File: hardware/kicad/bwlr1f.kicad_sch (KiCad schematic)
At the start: 68 parts, among them J1 Conn_01x02, Q2 PMV32UP, Q3 DMG1012UW, U1 BME688, U1 RAK3172-SIP, U2 NBM7100ABQX, U3 ZD24C08A, U5 TPL5110

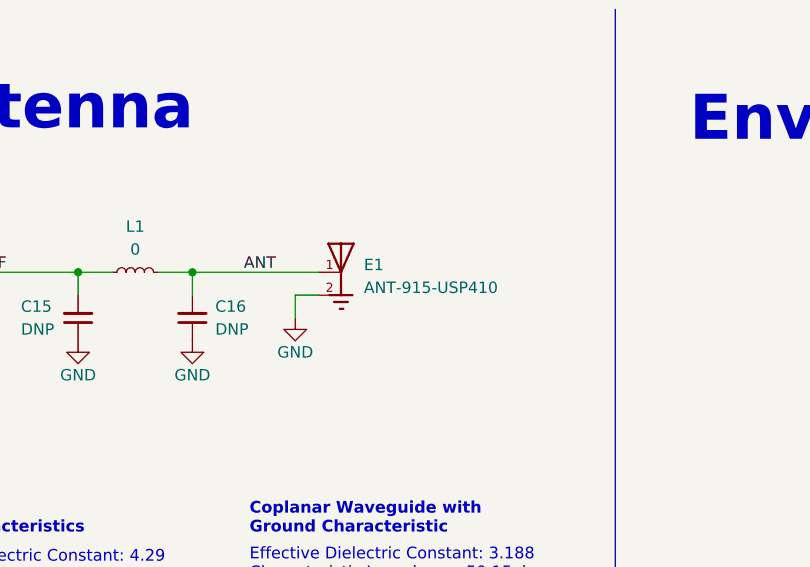
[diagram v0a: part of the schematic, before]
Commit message: change antenna
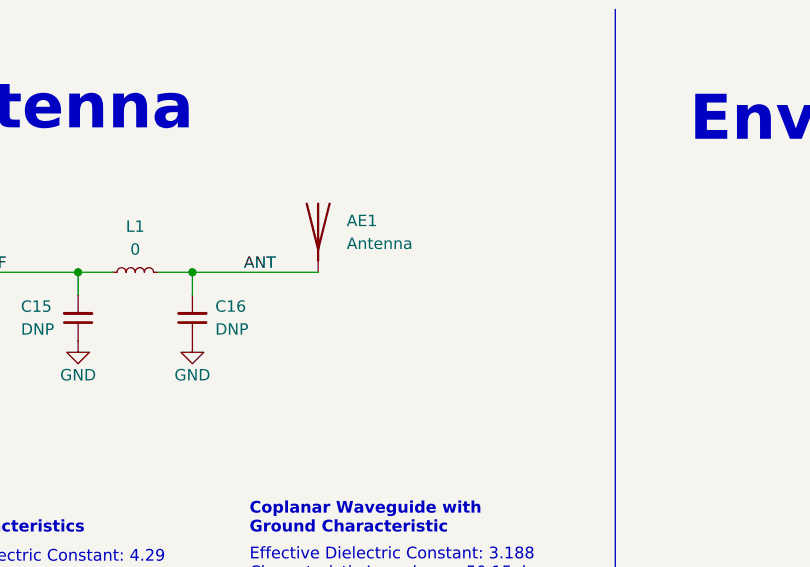
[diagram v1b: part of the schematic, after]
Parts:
- removed E1: ANT-915-USP410, bwlr1f:XDCR_ANT-915-USP410, symbol bwlr1f:ANT-915-USP410
- added AE1: Antenna, RF_Antenna:Texas_SWRA416_868MHz_915MHz, symbol Device:Antenna
- C15, C16: footprint Capacitor_SMD:C_0603_1608Metric -> Capacitor_SMD:C_0402_1005Metric
- L1: footprint Inductor_SMD:L_0603_1608Metric -> Inductor_SMD:L_0402_1005Metric; Distributor LCSC -> (none); Distributor Link https://www.lcsc.com/product-detail/Chip-Resistor-Surface-M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 -> (none); Distributor Part Number C21189 -> (none); Manufacturer UNI-ROYAL(Uniroyal Elec) -> (none); Manufacturer Part Number 0603WAF0000T5E -> (none); Part Description Resistors 100mW 75V ±1% 0Ω -> (none)
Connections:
- net ANT: now also AE1.1 (A)
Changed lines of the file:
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@@
     (stroke (width 0) (type default))
   )
-  (wire (pts (xy 243.84 45.72) (xy 243.84 43.18))
-    (stroke (width 0) (type default))
-  )
   (wire (pts (xy 44.45 43.18) (xy 44.45 41.91))
     (stroke (width 0) (type default))
   )
-  (wire (pts (xy 243.84 43.18) (xy 246.38 43.18))
-    (stroke (width 0) (type default))
-  )
   (wire (pts (xy 350.52 51.435) (xy 351.79 51.435))
     (stroke (width 0) (type default))
@@
     )
   )
+  (symbol (lib_id "Device:Antenna") (at 246.38 35.56 0) (unit 1)
+    (in_bom yes) (on_board yes) (dnp no) (fields_autoplaced)
+    (property "Reference" "AE1" (at 249.555 34.925 0)
+      (effects (font (size 1.27 1.27)) (justify left))
+    )
+    (property "Value" "Antenna" (at 249.555 37.465 0)
+      (effects (font (size 1.27 1.27)) (justify left))
+    )
+    (property "Footprint" "RF_Antenna:Texas_SWRA416_868MHz_915MHz" (at 246.38 35.56 0)
+      (effects (font (size 1.27 1.27)) hide)
+    )
+    (property "Datasheet" "~" (at 246.38 35.56 0)
+      (effects (font (size 1.27 1.27)) hide)
+    )
+    (property "Part Description" "" (at 246.38 35.56 0)
+      (effects (font (size 1.27 1.27)) hide)
+    )
+    (property "Manufacturer" "" (at 246.38 35.56 0)
+      (effects (font (size 1.27 1.27)) hide)
+    )
+    (property "Manufacturer Part Number" "" (at 246.38 35.56 0)
+      (effects (font (size 1.27 1.27)) hide)
+    )
+    (property "Distributor" "" (at 246.38 35.56 0)
+      (effects (font (size 1.27 1.27)) hide)
+    )
+    (property "Distributor Part Number" "" (at 246.38 35.56 0)
+      (effects (font (size 1.27 1.27)) hide)
+    )
+    (property "Distributor Link" "" (at 246.38 35.56 0)
+      (effects (font (size 1.27 1.27)) hide)
+    )
+    (pin "1")
+    (instances
+      (project "bwlr1f"
+        (path "/7fec048a-2dfd-4bff-8685-e805b00dfe07"
+          (reference "AE1") (unit 1)
+        )
+      )
+    )
+  )
   (symbol (lib_id "Device:C_Small") (at 232.41 45.72 180) (unit 1)
     (in_bom yes) (on_board yes) (dnp no) (fields_autoplaced)
@@
       (effects (font (size 1.27 1.27)) (justify right))
     )
-    (property "Footprint" "Capacitor_SMD:C_0603_1608Metric" (at 232.41 45.72 0)
+    (property "Footprint" "Capacitor_SMD:C_0402_1005Metric" (at 232.41 45.72 0)
       (effects (font (size 1.27 1.27)) hide)
     )
@@
       (effects (font (size 1.27 1.27)) hide)
     )
+    (property "Part Description" "" (at 232.41 45.72 0)
+      (effects (font (size 1.27 1.27)) hide)
+    )
+    (property "Manufacturer" "" (at 232.41 45.72 0)
+      (effects (font (size 1.27 1.27)) hide)
+    )
+    (property "Distributor" "" (at 232.41 45.72 0)
+      (effects (font (size 1.27 1.27)) hide)
+    )
+    (property "Distributor Part Number" "" (at 232.41 45.72 0)
+      (effects (font (size 1.27 1.27)) hide)
+    )
+    (property "Distributor Link" "" (at 232.41 45.72 0)
+      (effects (font (size 1.27 1.27)) hide)
+    )
     (pin "1")
     (pin "2")
@@
       (effects (font (size 1.27 1.27)))
     )
-    (property "Footprint" "Inductor_SMD:L_0603_1608Metric" (at 226.06 40.64 0)
-      (effects (font (size 1.27 1.27)) hide)
-    )
-    (property "Datasheet" "https://datasheet.lcsc.com/lcsc/2206010130_UNI-ROYAL-Uniroyal-Elec-0603WAF0000T5E_C21189.pdf" (at 226.06 40.64 0)
+    (property "Footprint" "Inductor_SMD:L_0402_1005Metric" (at 226.06 40.64 0)
       (effects (font (size 1.27 1.27)) hide)
     )
-    (property "Manufacturer Part Number" "0603WAF0000T5E" (at 226.06 40.64 0)
-      (effects (font (size 1.27 1.27)) hide)
-    )
-    (property "Part Description" "Resistors 100mW 75V ±1% 0Ω" (at 226.06 40.64 0)
-      (effects (font (size 1.27 1.27)) hide)
-    )
-    (property "Manufacturer" "UNI-ROYAL(Uniroyal Elec)" (at 226.06 40.64 0)
-      (effects (font (size 1.27 1.27)) hide)
-    )
-    (property "Distributor" "LCSC" (at 226.06 40.64 0)
-      (effects (font (size 1.27 1.27)) hide)
-    )
-    (property "Distributor Part Number" "C21189" (at 226.06 40.64 0)
-      (effects (font (size 1.27 1.27)) hide)
-    )
-    (property "Distributor Link" "https://www.lcsc.com/product-detail/Chip-Resistor-Surface-Mount_UNI-ROYAL-Uniroyal-Elec-0603WAF0000T5E_C21189.html" (at 226.06 40.64 0)
+    (property "Datasheet" "" (at 226.06 40.64 0)
       (effects (font (size 1.27 1.27)) hide)
     )
@@
       (effects (font (size 1.27 1.27)) (justify right))
     )
-    (property "Footprint" "Capacitor_SMD:C_0603_1608Metric" (at 219.71 45.72 0)
+    (property "Footprint" "Capacitor_SMD:C_0402_1005Metric" (at 219.71 45.72 0)
       (effects (font (size 1.27 1.27)) hide)
     )
@@
     )
   )
-  (symbol (lib_id "bwlr1f:ANT-915-USP410") (at 248.92 40.64 0) (unit 1)
-    (in_bom yes) (on_board yes) (dnp no) (fields_autoplaced)
-    (property "Reference" "E1" (at 251.46 39.8145 0)
-      (effects (font (size 1.27 1.27)) (justify left))
-    )
-    (property "Value" "ANT-915-USP410" (at 251.46 42.3545 0)
-      (effects (font (size 1.27 1.27)) (justify left))
-    )
-    (property "Footprint" "bwlr1f:XDCR_ANT-915-USP410" (at 243.84 50.8 0)
-      (effects (font (size 1.27 1.27)) (justify left bottom) hide)
-    )
-    (property "Datasheet" "https://www.te.com/commerce/DocumentDelivery/DDEController?Action=srchrtrv&DocNm=ant-915-usp410-ds&DocType=Data+Sheet&DocLang=English&DocFormat=pdf&PartCntxt=ANT-915-USP410" (at 248.92 40.64 0)
-      (effects (font (size 1.27 1.27)) (justify left bottom) hide)
-    )
-    (property "Part Description" "915MHz ISM, LoRaWAN, LPWA, Sigfox Chip RF Antenna 902MHz ~ 930MHz 0.9dBi Solder Surface Mount" (at 248.92 40.64 0)
-      (effects (font (size 1.27 1.27)) hide)
-    )
-    (property "Manufacturer" "TE Connectivity Linx" (at 248.92 40.64 0)
-      (effects (font (size 1.27 1.27)) hide)
-    )
-    (property "Manufacturer Part Number" "ANT-915-USP410" (at 248.92 40.64 0)
-      (effects (font (size 1.27 1.27)) hide)
-    )
-    (property "Distributor" "Digikey" (at 248.92 40.64 0)
-      (effects (font (size 1.27 1.27)) hide)
-    )
-    (property "Distributor Part Number" "343-ANT-915-USP410CT-ND" (at 248.92 40.64 0)
-      (effects (font (size 1.27 1.27)) hide)
-    )
-    (property "Distributor Link" "https://www.digikey.com/en/products/detail/te-connectivity-linx/ANT-915-USP410/13165344" (at 248.92 40.64 0)
-      (effects (font (size 1.27 1.27)) hide)
-    )
-    (pin "1")
-    (pin "2")
-    (instances
-      (project "bwlr1f"
-        (path "/7fec048a-2dfd-4bff-8685-e805b00dfe07"
-          (reference "E1") (unit 1)
-        )
-      )
-    )
-  )
   (symbol (lib_id "power:+3V0") (at 33.655 83.82 0) (unit 1)
     (in_bom yes) (on_board yes) (dnp no) (fields_autoplaced)
@@
         )
       )
-    )
-  )
-  (symbol (lib_id "power:GND") (at 243.84 45.72 0) (unit 1)
-    (in_bom yes) (on_board yes) (dnp no)
-    (property "Reference" "#PWR030" (at 243.84 52.07 0)
-      (effects (font (size 1.27 1.27)) hide)
-    )
-    (property "Value" "GND" (at 243.84 49.53 0)
-      (effects (font (size 1.27 1.27)))
-    )
-    (property "Footprint" "" (at 243.84 45.72 0)
-      (effects (font (size 1.27 1.27)) hide)
-    )
-    (property "Datasheet" "" (at 243.84 45.72 0)
-      (effects (font (size 1.27 1.27)) hide)
-    )
-    (pin "1")
-    (instances
-      (project "bwlr1e"
-        (path "/630c8da6-5464-4eef-824d-89618087f4b4"
-          (reference "#PWR030") (unit 1)
-        )
-      )
-      (project "bwlr1f"
-        (path "/7fec048a-2dfd-4bff-8685-e805b00dfe07"
-          (reference "#PWR038") (unit 1)
-        )
-      )

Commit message: Revert "change antenna"
This reverts commit 46c20b2a2dd1e0a5efdce99ceacd3ab7d772dc0d.
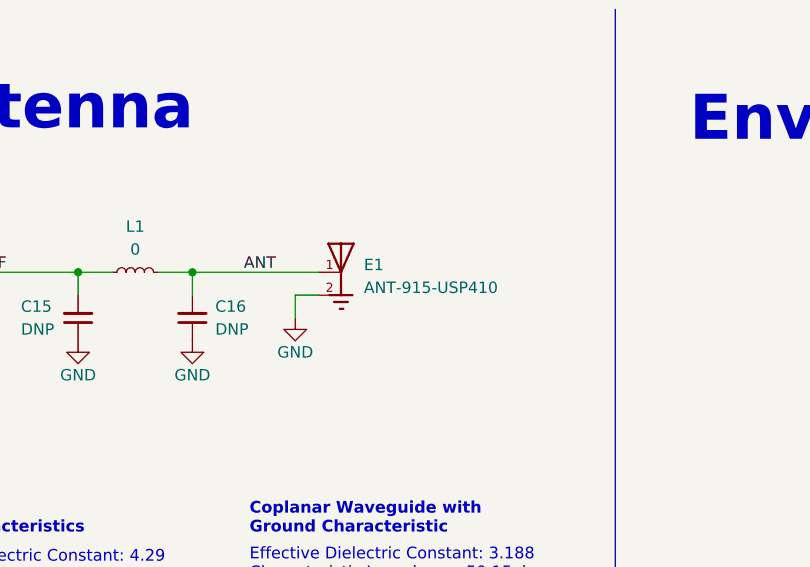
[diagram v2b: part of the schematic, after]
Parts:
- removed AE1: Antenna, RF_Antenna:Texas_SWRA416_868MHz_915MHz, symbol Device:Antenna
- added E1: ANT-915-USP410, bwlr1f:XDCR_ANT-915-USP410, symbol bwlr1f:ANT-915-USP410
- C15, C16: footprint Capacitor_SMD:C_0402_1005Metric -> Capacitor_SMD:C_0603_1608Metric
- L1: footprint Inductor_SMD:L_0402_1005Metric -> Inductor_SMD:L_0603_1608Metric; Distributor (none) -> LCSC; Distributor Link (none) -> https://www.lcsc.com/product-detail/Chip-Resistor-Surface-M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; Distributor Part Number (none) -> C21189; Manufacturer (none) -> UNI-ROYAL(Uniroyal Elec); Manufacturer Part Number (none) -> 0603WAF0000T5E; Part Description (none) -> Resistors 100mW 75V ±1% 0Ω
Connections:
- net ANT: now also E1.1
- net GND: now also E1.2
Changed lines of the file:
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@@
     (stroke (width 0) (type default))
   )
+  (wire (pts (xy 243.84 45.72) (xy 243.84 43.18))
+    (stroke (width 0) (type default))
+  )
   (wire (pts (xy 44.45 43.18) (xy 44.45 41.91))
     (stroke (width 0) (type default))
   )
+  (wire (pts (xy 243.84 43.18) (xy 246.38 43.18))
+    (stroke (width 0) (type default))
+  )
   (wire (pts (xy 350.52 51.435) (xy 351.79 51.435))
     (stroke (width 0) (type default))
@@
     )
   )
-  (symbol (lib_id "Device:Antenna") (at 246.38 35.56 0) (unit 1)
-    (in_bom yes) (on_board yes) (dnp no) (fields_autoplaced)
-    (property "Reference" "AE1" (at 249.555 34.925 0)
-      (effects (font (size 1.27 1.27)) (justify left))
-    )
-    (property "Value" "Antenna" (at 249.555 37.465 0)
-      (effects (font (size 1.27 1.27)) (justify left))
-    )
-    (property "Footprint" "RF_Antenna:Texas_SWRA416_868MHz_915MHz" (at 246.38 35.56 0)
-      (effects (font (size 1.27 1.27)) hide)
-    )
-    (property "Datasheet" "~" (at 246.38 35.56 0)
-      (effects (font (size 1.27 1.27)) hide)
-    )
-    (property "Part Description" "" (at 246.38 35.56 0)
-      (effects (font (size 1.27 1.27)) hide)
-    )
-    (property "Manufacturer" "" (at 246.38 35.56 0)
-      (effects (font (size 1.27 1.27)) hide)
-    )
-    (property "Manufacturer Part Number" "" (at 246.38 35.56 0)
-      (effects (font (size 1.27 1.27)) hide)
-    )
-    (property "Distributor" "" (at 246.38 35.56 0)
-      (effects (font (size 1.27 1.27)) hide)
-    )
-    (property "Distributor Part Number" "" (at 246.38 35.56 0)
-      (effects (font (size 1.27 1.27)) hide)
-    )
-    (property "Distributor Link" "" (at 246.38 35.56 0)
-      (effects (font (size 1.27 1.27)) hide)
-    )
-    (pin "1")
-    (instances
-      (project "bwlr1f"
-        (path "/7fec048a-2dfd-4bff-8685-e805b00dfe07"
-          (reference "AE1") (unit 1)
-        )
-      )
-    )
-  )
   (symbol (lib_id "Device:C_Small") (at 232.41 45.72 180) (unit 1)
     (in_bom yes) (on_board yes) (dnp no) (fields_autoplaced)
@@
       (effects (font (size 1.27 1.27)) (justify right))
     )
-    (property "Footprint" "Capacitor_SMD:C_0402_1005Metric" (at 232.41 45.72 0)
+    (property "Footprint" "Capacitor_SMD:C_0603_1608Metric" (at 232.41 45.72 0)
       (effects (font (size 1.27 1.27)) hide)
     )
@@
       (effects (font (size 1.27 1.27)) hide)
     )
-    (property "Part Description" "" (at 232.41 45.72 0)
-      (effects (font (size 1.27 1.27)) hide)
-    )
-    (property "Manufacturer" "" (at 232.41 45.72 0)
-      (effects (font (size 1.27 1.27)) hide)
-    )
-    (property "Distributor" "" (at 232.41 45.72 0)
-      (effects (font (size 1.27 1.27)) hide)
-    )
-    (property "Distributor Part Number" "" (at 232.41 45.72 0)
-      (effects (font (size 1.27 1.27)) hide)
-    )
-    (property "Distributor Link" "" (at 232.41 45.72 0)
-      (effects (font (size 1.27 1.27)) hide)
-    )
     (pin "1")
     (pin "2")
@@
       (effects (font (size 1.27 1.27)))
     )
-    (property "Footprint" "Inductor_SMD:L_0402_1005Metric" (at 226.06 40.64 0)
+    (property "Footprint" "Inductor_SMD:L_0603_1608Metric" (at 226.06 40.64 0)
+      (effects (font (size 1.27 1.27)) hide)
+    )
+    (property "Datasheet" "https://datasheet.lcsc.com/lcsc/2206010130_UNI-ROYAL-Uniroyal-Elec-0603WAF0000T5E_C21189.pdf" (at 226.06 40.64 0)
       (effects (font (size 1.27 1.27)) hide)
     )
-    (property "Datasheet" "" (at 226.06 40.64 0)
+    (property "Manufacturer Part Number" "0603WAF0000T5E" (at 226.06 40.64 0)
+      (effects (font (size 1.27 1.27)) hide)
+    )
+    (property "Part Description" "Resistors 100mW 75V ±1% 0Ω" (at 226.06 40.64 0)
+      (effects (font (size 1.27 1.27)) hide)
+    )
+    (property "Manufacturer" "UNI-ROYAL(Uniroyal Elec)" (at 226.06 40.64 0)
+      (effects (font (size 1.27 1.27)) hide)
+    )
+    (property "Distributor" "LCSC" (at 226.06 40.64 0)
+      (effects (font (size 1.27 1.27)) hide)
+    )
+    (property "Distributor Part Number" "C21189" (at 226.06 40.64 0)
+      (effects (font (size 1.27 1.27)) hide)
+    )
+    (property "Distributor Link" "https://www.lcsc.com/product-detail/Chip-Resistor-Surface-Mount_UNI-ROYAL-Uniroyal-Elec-0603WAF0000T5E_C21189.html" (at 226.06 40.64 0)
       (effects (font (size 1.27 1.27)) hide)
     )
@@
       (effects (font (size 1.27 1.27)) (justify right))
     )
-    (property "Footprint" "Capacitor_SMD:C_0402_1005Metric" (at 219.71 45.72 0)
+    (property "Footprint" "Capacitor_SMD:C_0603_1608Metric" (at 219.71 45.72 0)
       (effects (font (size 1.27 1.27)) hide)
     )
@@
     )
   )
+  (symbol (lib_id "bwlr1f:ANT-915-USP410") (at 248.92 40.64 0) (unit 1)
+    (in_bom yes) (on_board yes) (dnp no) (fields_autoplaced)
+    (property "Reference" "E1" (at 251.46 39.8145 0)
+      (effects (font (size 1.27 1.27)) (justify left))
+    )
+    (property "Value" "ANT-915-USP410" (at 251.46 42.3545 0)
+      (effects (font (size 1.27 1.27)) (justify left))
+    )
+    (property "Footprint" "bwlr1f:XDCR_ANT-915-USP410" (at 243.84 50.8 0)
+      (effects (font (size 1.27 1.27)) (justify left bottom) hide)
+    )
+    (property "Datasheet" "https://www.te.com/commerce/DocumentDelivery/DDEController?Action=srchrtrv&DocNm=ant-915-usp410-ds&DocType=Data+Sheet&DocLang=English&DocFormat=pdf&PartCntxt=ANT-915-USP410" (at 248.92 40.64 0)
+      (effects (font (size 1.27 1.27)) (justify left bottom) hide)
+    )
+    (property "Part Description" "915MHz ISM, LoRaWAN, LPWA, Sigfox Chip RF Antenna 902MHz ~ 930MHz 0.9dBi Solder Surface Mount" (at 248.92 40.64 0)
+      (effects (font (size 1.27 1.27)) hide)
+    )
+    (property "Manufacturer" "TE Connectivity Linx" (at 248.92 40.64 0)
+      (effects (font (size 1.27 1.27)) hide)
+    )
+    (property "Manufacturer Part Number" "ANT-915-USP410" (at 248.92 40.64 0)
+      (effects (font (size 1.27 1.27)) hide)
+    )
+    (property "Distributor" "Digikey" (at 248.92 40.64 0)
+      (effects (font (size 1.27 1.27)) hide)
+    )
+    (property "Distributor Part Number" "343-ANT-915-USP410CT-ND" (at 248.92 40.64 0)
+      (effects (font (size 1.27 1.27)) hide)
+    )
+    (property "Distributor Link" "https://www.digikey.com/en/products/detail/te-connectivity-linx/ANT-915-USP410/13165344" (at 248.92 40.64 0)
+      (effects (font (size 1.27 1.27)) hide)
+    )
+    (pin "1")
+    (pin "2")
+    (instances
+      (project "bwlr1f"
+        (path "/7fec048a-2dfd-4bff-8685-e805b00dfe07"
+          (reference "E1") (unit 1)
+        )
+      )
+    )
+  )
   (symbol (lib_id "power:+3V0") (at 33.655 83.82 0) (unit 1)
     (in_bom yes) (on_board yes) (dnp no) (fields_autoplaced)
@@
         )
       )
+    )
+  )
+  (symbol (lib_id "power:GND") (at 243.84 45.72 0) (unit 1)
+    (in_bom yes) (on_board yes) (dnp no)
+    (property "Reference" "#PWR030" (at 243.84 52.07 0)
+      (effects (font (size 1.27 1.27)) hide)
+    )
+    (property "Value" "GND" (at 243.84 49.53 0)
+      (effects (font (size 1.27 1.27)))
+    )
+    (property "Footprint" "" (at 243.84 45.72 0)
+      (effects (font (size 1.27 1.27)) hide)
+    )
+    (property "Datasheet" "" (at 243.84 45.72 0)
+      (effects (font (size 1.27 1.27)) hide)
+    )
+    (pin "1")
+    (instances
+      (project "bwlr1e"
+        (path "/630c8da6-5464-4eef-824d-89618087f4b4"
+          (reference "#PWR030") (unit 1)
+        )
+      )
+      (project "bwlr1f"
+        (path "/7fec048a-2dfd-4bff-8685-e805b00dfe07"
+          (reference "#PWR038") (unit 1)
+        )
+      )
